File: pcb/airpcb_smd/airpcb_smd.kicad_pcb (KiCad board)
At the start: 2 copper layers, 49.5 x 40.6 mm, 34 parts, among them J1 SPI, J11 PSU, J2 DHT, J3 DC, J4 AB, J5 Conn_01x08, J6 Conn_01x08, J7 PWR, J8 WS2812, J9 5V3V, Q1 PN2222A, Q2 PN2222A, U1 PC817, U2 PC817, U3 WeMos_D1_mini, U4 ESP-12E

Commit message: feat(pcb kicad project): update to v6 * migrated to kicad v6
* added nodemcu symbols & footprints ( nodemcu project lib )

Signed-off-by: Jose Vega <josevega234@gmail.com>
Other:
- net class Default removed

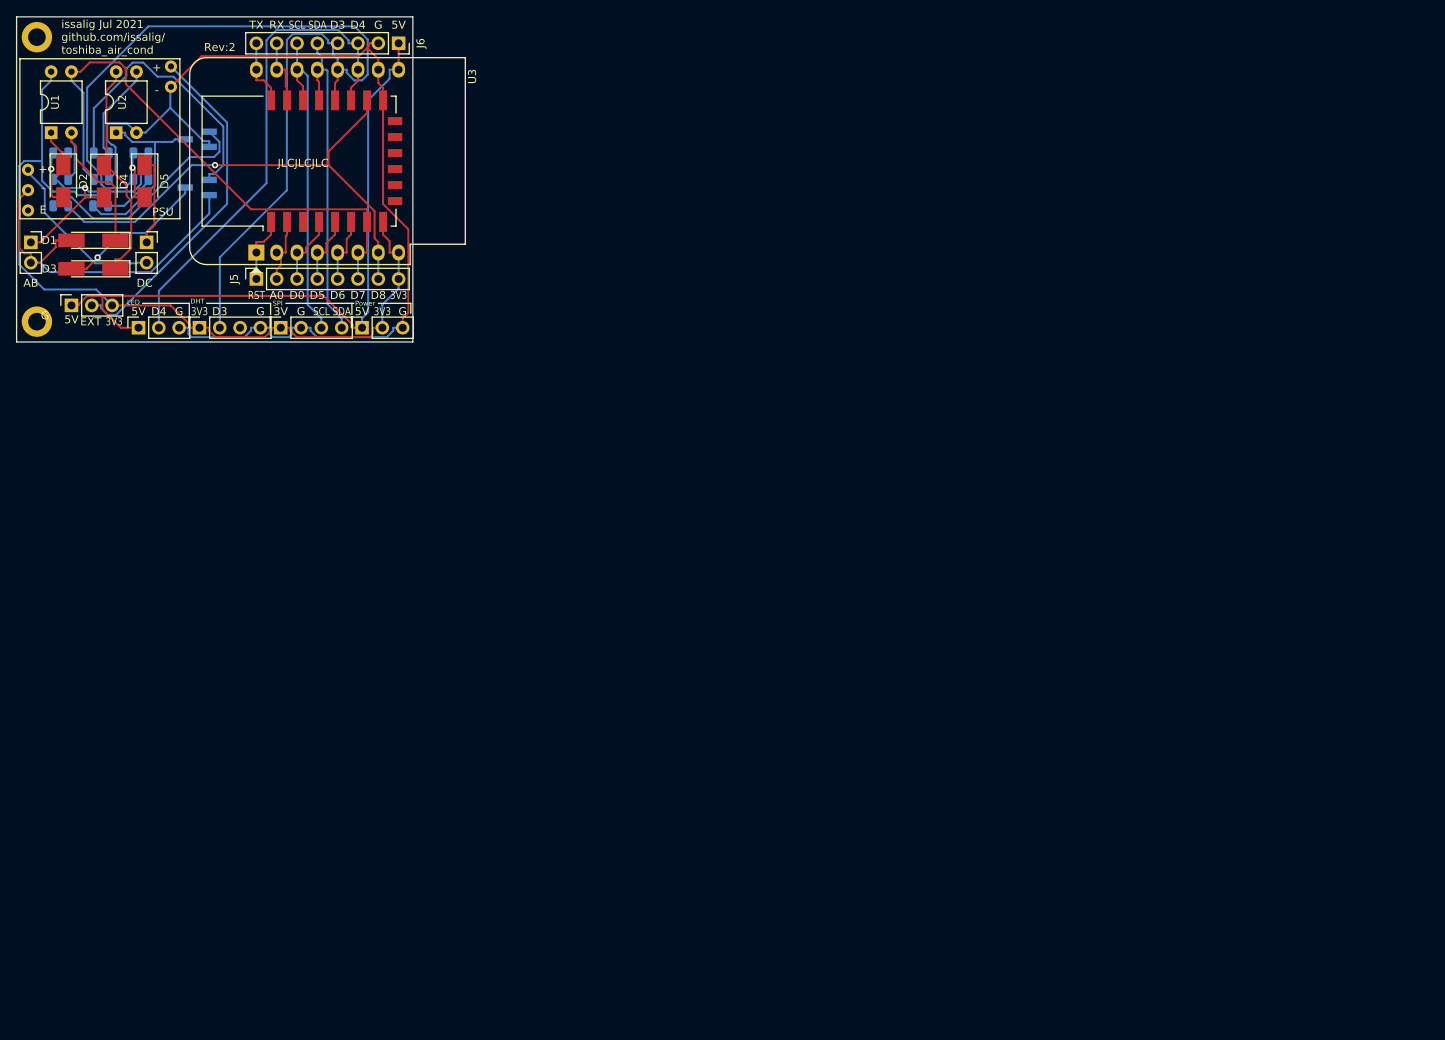
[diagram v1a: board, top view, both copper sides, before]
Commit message: routing
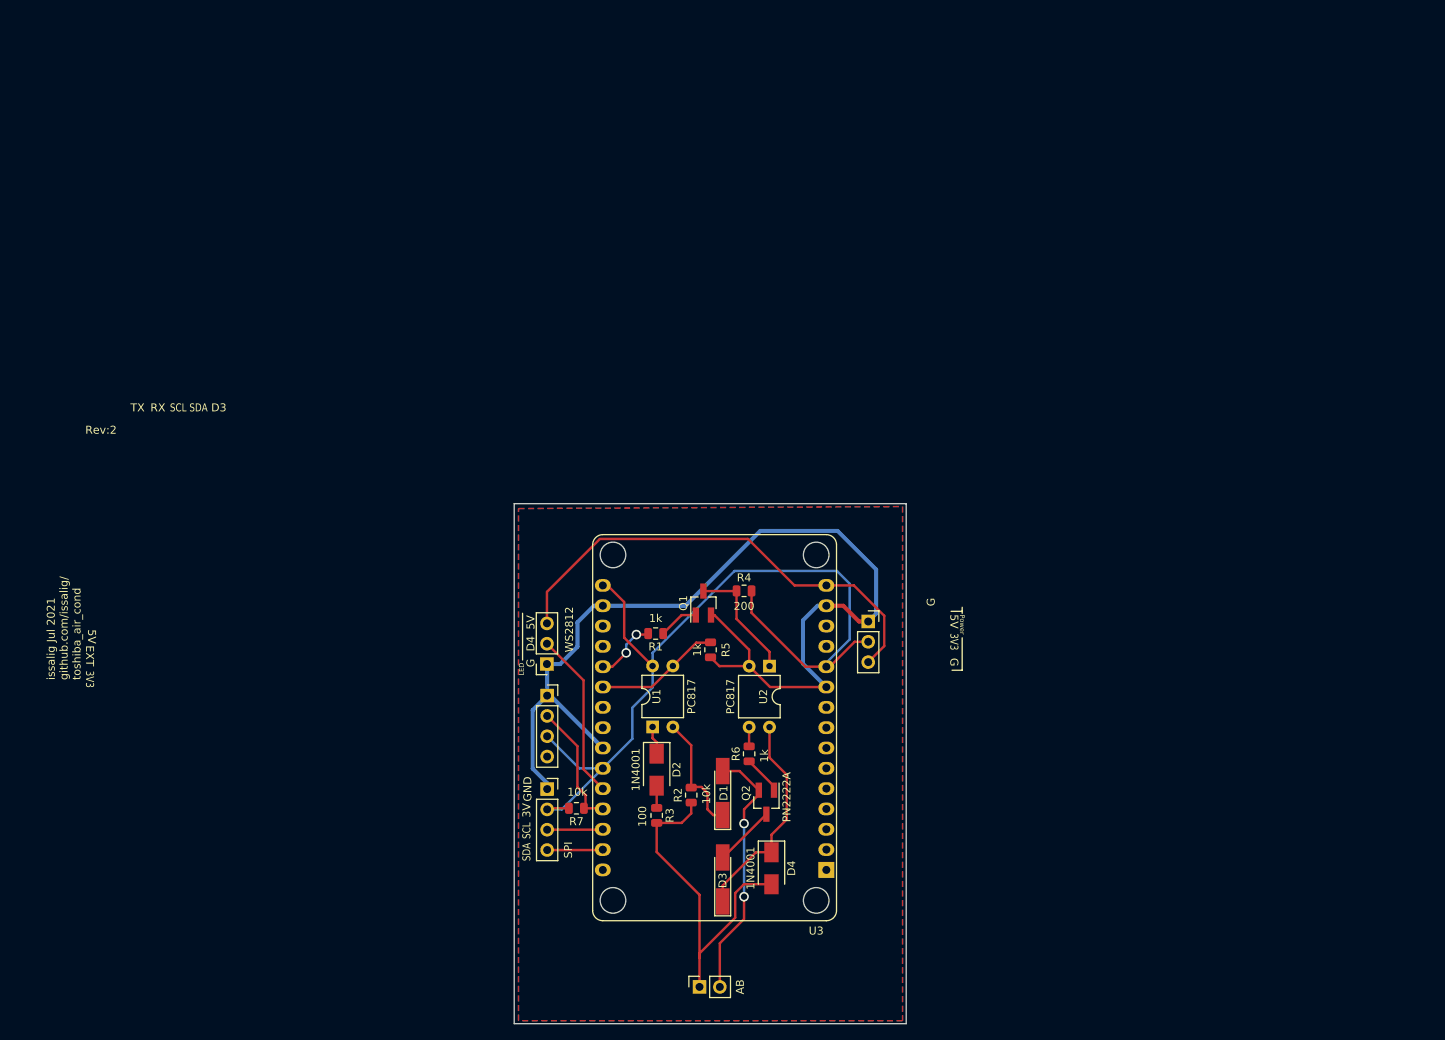
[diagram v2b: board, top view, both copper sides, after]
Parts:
- removed D5: 1N4001, Diode_SMD:D_SMA
- removed J11: PSU, airpcb_smd:HW-108
- removed J3: DC, Connector_PinSocket_2.54mm:PinSocket_1x02_P2.54mm_Vertical
- removed J5, J6: Conn_01x08, Connector_PinSocket_2.54mm:PinSocket_1x08_P2.54mm_Vertical
- removed J9: 5V3V, Connector_PinSocket_2.54mm:PinSocket_1x03_P2.54mm_Vertical
- removed L1: KiCad-Logo2_5mm_SilkScreen, Symbol:KiCad-Logo2_5mm_SilkScreen
- removed L2: OSHW-Logo2_7.3x6mm_SilkScreen, Symbol:OSHW-Logo2_7.3x6mm_SilkScreen
- removed L3: WEEE-Logo_4.2x6mm_SilkScreen, Symbol:WEEE-Logo_4.2x6mm_SilkScreen
- removed M1, M2: , MountingHole:MountingHole_2.2mm_M2_DIN965_Pad
- removed R8: 100, Resistor_SMD:R_0805_2012Metric
- removed U4: ESP-12E, RF_Module:ESP-12E
- Q1, Q2, R1, R2, R3, R4, R5, R6, R7: moved to F.Cu
- U3: value WeMos_D1_mini -> NodeMCU_ESP-12E; footprint Module:WEMOS_D1_mini_light -> nodemcu:NodeMCU_ESP-12E_WithMountingHoles
- moved J4 125.1 mm to (136.2, 130.4), turned to 90 degrees
- moved D4 119.7 mm to (145.2, 115.6)
- moved R3 111.4 mm to (130.8, 109.0), turned to -90 degrees
- moved R6 110.4 mm to (142.4, 101.3), turned to 90 degrees
- moved R2 110.2 mm to (135.1, 106.4), turned to 90 degrees
- moved D3 109.6 mm to (139.1, 117.0), turned to 90 degrees
- moved U1 105.7 mm to (130.3, 97.9)
- moved U2 105.4 mm to (144.9, 90.3), turned to -90 degrees
- moved U3 105.0 mm to (152.0, 115.8), turned to 180 degrees
- moved Q2 104.7 mm to (144.5, 107.3), turned to -90 degrees
- moved D1 104.7 mm to (139.1, 106.2), turned to 90 degrees
- moved D2 104.5 mm to (130.8, 103.3)
- moved R5 96.2 mm to (137.5, 88.3), turned to -90 degrees
- moved R7 95.6 mm to (120.8, 108.1), turned to 180 degrees
- moved R4 93.7 mm to (141.7, 80.9)
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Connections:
- J1 pad 1: 3V3 -> GND
- J1 pad 2: GND -> 3V3
- J2 pad 1: 3V3 -> GND
- J2 pad 3: Net-(J2-Pad3) -> 3V3
- J2 pad 4: GND -> unconnected-(J2-Pad4)
- J7 pad 1: 5V -> GND
- J7 pad 3: GND -> 5V
- J8 pad 1: 5V -> GND
- J8 pad 3: GND -> 5V
- U3 pad 1: RST -> unconnected-(U3-Pad1)
- U3 pad 11: D4 -> 3V3
- U3 pad 12: D3 -> unconnected-(U3-Pad12)
- U3 pad 13: SDA -> RST
- U3 pad 14: SCL -> GND
- U3 pad 15: ESP_RX -> 5V
- U3 pad 16: ESP_TX -> 3V3
- U3 pad 3: D0 -> unconnected-(U3-Pad3)
- U3 pad 4: D5 -> unconnected-(U3-Pad4)
- U3 pad 5: D6 -> unconnected-(U3-Pad5)
- U3 pad 6: D7 -> unconnected-(U3-Pad6)
- U3 pad 7: D8 -> unconnected-(U3-Pad7)
- U3 pad 8: 3V3 -> unconnected-(U3-Pad8)
- U3 pad 9: 5V -> unconnected-(U3-Pad9)
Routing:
- net D3: track 119.9 -> 16.0 mm
- net D8: track 63.2 -> 7.98 mm, vias 1 -> 2
- net D7: track 70.6 -> 15.8 mm
- net PSU_OUT: track 43.4 -> 0.00 mm
- net D4: track 61.9 -> 21.0 mm
- net SDA: track 41.6 -> 6.98 mm
- net SCL: track 41.5 -> 6.98 mm
- net Net-(Q2-Pad2): track 35.7 -> 4.90 mm
- net 5V: track 84.0 -> 59.4 mm
- net Net-(Q1-Pad2): track 28.8 -> 5.04 mm
- net Net-(J11-Pad3): track 21.6 -> 0.00 mm
- net B: track 45.5 -> 32.1 mm, vias 0 -> 2
- net Net-(D5-Pad1): track 11.3 -> 0.00 mm
- net Net-(D3-Pad2): track 18.9 -> 7.70 mm, vias 1 -> 0
- net A: track 32.9 -> 43.8 mm, vias 1 -> 0
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- added copper zone on B.Cu, net 3V3
- added copper zone on F.Cu, net 3V3
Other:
- board size 49.5 x 40.6 mm -> 49 x 65 mm
- board text added: "GND"
- board text removed: "+"
- board text removed: "-"
- board text removed: "A0"
- board text removed: "D0"
- board text removed: "D5"
- board text removed: "D6"
- board text removed: "D7"
- board text removed: "D8"
- board text removed: "DHT"
- board text removed: "E"
- board text removed: "FreeRouting powered"
- board text removed: "JLCJLCJLC"
- board text removed: "RST"
- board text removed: "SPI"

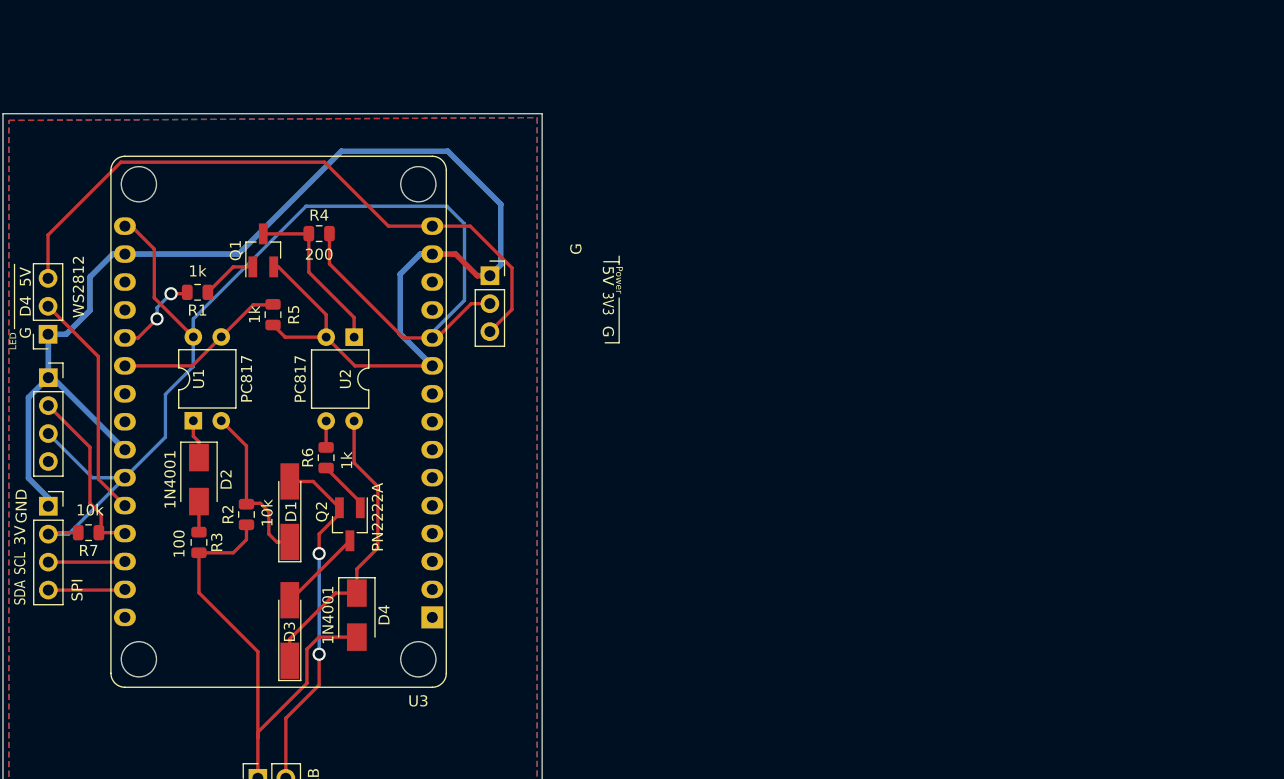
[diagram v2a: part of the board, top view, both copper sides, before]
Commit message: schematic done
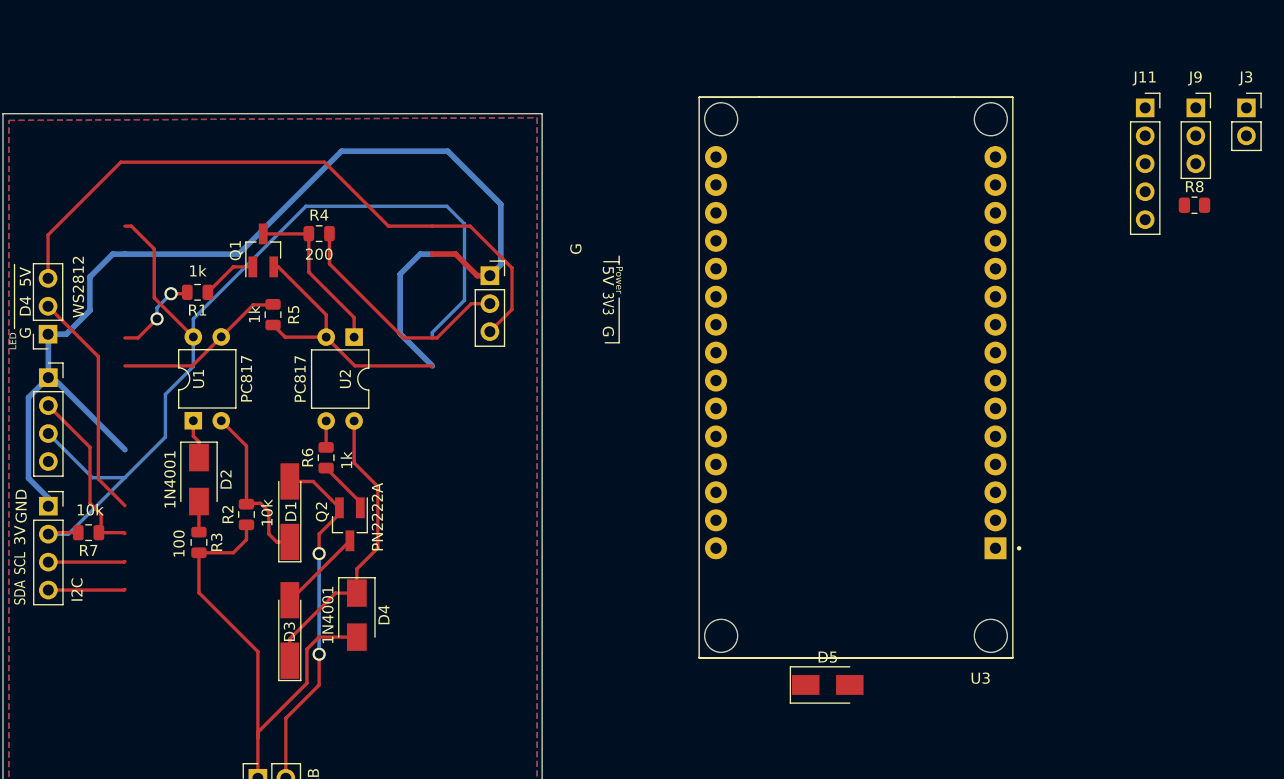
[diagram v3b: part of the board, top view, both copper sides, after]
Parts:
- added D5: 1N4001, Diode_SMD:D_SMA, F.Cu at (188.0, 121.9)
- added J11: PSU, Connector_PinSocket_2.54mm:PinSocket_1x05_P2.54mm_Vertical, F.Cu at (216.8, 69.5)
- added J3: DC, Connector_PinSocket_2.54mm:PinSocket_1x02_P2.54mm_Vertical, F.Cu at (226.0, 69.5)
- added J9: 5V3V, Connector_PinSocket_2.54mm:PinSocket_1x03_P2.54mm_Vertical, F.Cu at (221.4, 69.5)
- added R8: 100, Resistor_SMD:R_0805_2012Metric, F.Cu at (221.3, 78.3)
- J1: value SPI -> I2C
- U3: value NodeMCU_ESP-12E -> ESP32-DEVKIT-V1; footprint nodemcu:NodeMCU_ESP-12E_WithMountingHoles -> airpcb_smd:MODULE_ESP32_DEVKIT_V1
- moved U3 44.2 mm to (190.5, 94.0)
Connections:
- J2 pad 2: D3 -> D2
- R1 pad 2: D8 -> D13
- R5 pad 1: D7 -> D12
- R7 pad 1: D3 -> D2
- U1 pad 3: D7 -> D12
- U3 pad 1: unconnected-(U3-Pad1) -> 3V3
- U3 pad 10: GND -> unconnected-(U3-Pad10)
- U3 pad 11: 3V3 -> SDA
- U3 pad 13: RST -> unconnected-(U3-Pad13)
- U3 pad 14: GND -> SCL
- U3 pad 15: 5V -> unconnected-(U3-Pad15)
- U3 pad 16: 3V3 -> unconnected-(U3-Pad16)
- U3 pad 17: GND -> unconnected-(U3-Pad17)
- U3 pad 18: ESP_TX -> unconnected-(U3-Pad18)
- U3 pad 19: ESP_RX -> unconnected-(U3-Pad19)
- U3 pad 2: A0 -> GND
- U3 pad 20: D8 -> unconnected-(U3-Pad20)
- U3 pad 21: D7 -> unconnected-(U3-Pad21)
- U3 pad 22: D6 -> unconnected-(U3-Pad22)
- U3 pad 23: D5 -> unconnected-(U3-Pad23)
- U3 pad 24: GND -> unconnected-(U3-Pad24)
- U3 pad 25: 3V3 -> unconnected-(U3-Pad25)
- U3 pad 26: D4 -> unconnected-(U3-Pad26)
- U3 pad 27: D3 -> D12
- U3 pad 28: SCL -> D13
- U3 pad 29: SDA -> GND
- U3 pad 30: D0 -> 5V
- U3 pad 4: unconnected-(U3-Pad4) -> D2
- U3 pad 5: unconnected-(U3-Pad5) -> D4
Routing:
- net D3: track 16.0 -> 0.00 mm
- net D2: track 0.00 -> 16.0 mm
- net D7: track 15.8 -> 0.00 mm
- net D12: track 0.00 -> 15.8 mm
- net D8: track 7.98 -> 0.00 mm, vias 2 -> 0
- net D13: track 0.00 -> 7.98 mm, vias 0 -> 2
